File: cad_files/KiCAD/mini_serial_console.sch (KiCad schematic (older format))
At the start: 45 parts, among them J1 Screw_Terminal_1x02, J2 Screw_Terminal_1x03, J3 Screw_Terminal_1x03, J4 Screw_Terminal_1x07, Q1 BC559, Q2 BC548, Q3 BC109, U1 HD44780 compatible LCD, U2 Raspberry Pi Pico

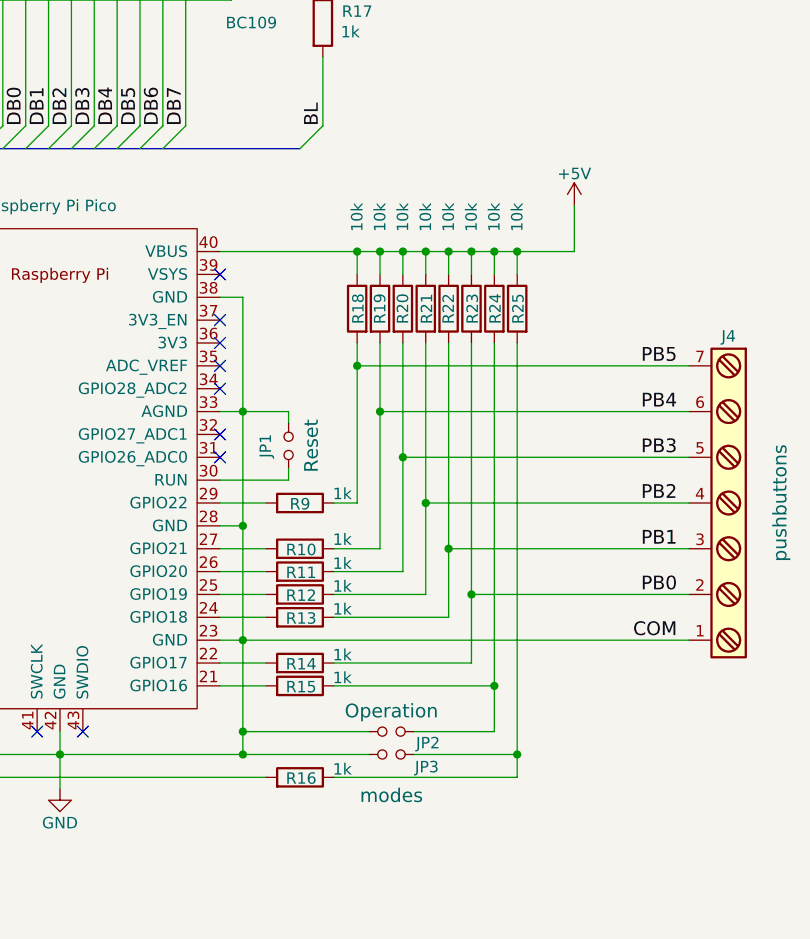
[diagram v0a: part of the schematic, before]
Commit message: 221115
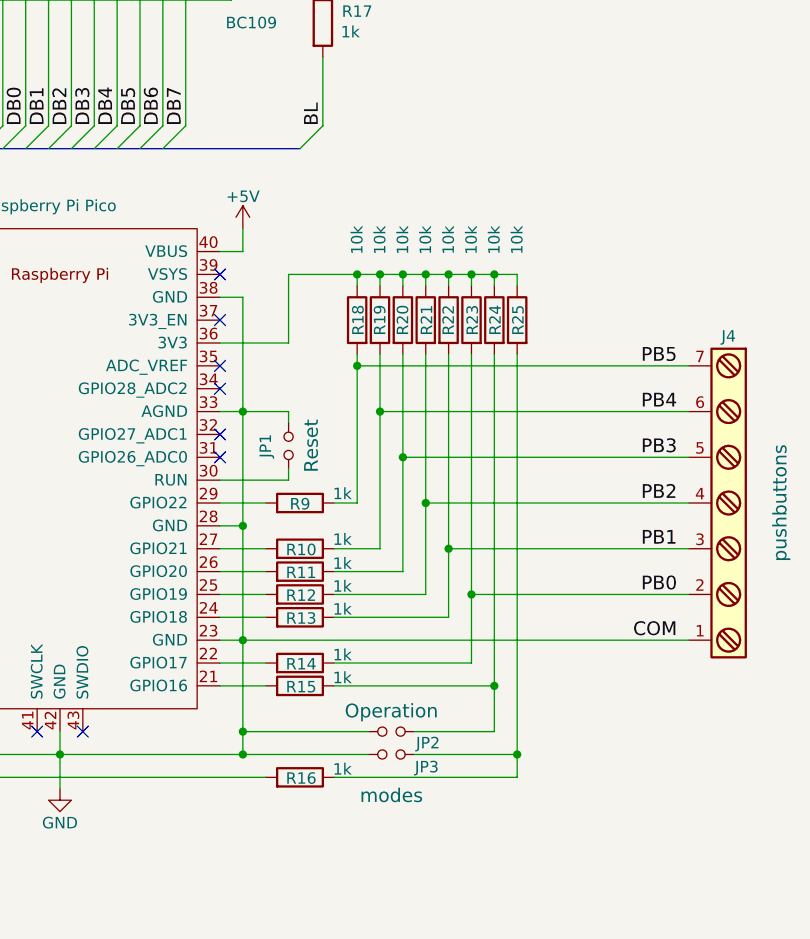
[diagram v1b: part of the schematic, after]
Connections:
- net +5V: no longer R18.1, R19.1, R20.1, R21.1, R22.1, R23.1, R24.1, R25.1
- net at U2.36 (3V3): now also R18.1, R19.1, R20.1, R21.1, R22.1, R23.1, R24.1, R25.1
- no-connect marks 9 -> 8
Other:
- moved on the sheet: R18, R19, R20, R21, R22, R23, R24, R25
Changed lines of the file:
@@
 Entry Wire Line
 	6300 3300 6400 3200
-NoConn ~ 7550 4150
 NoConn ~ 7550 4050
 NoConn ~ 7550 3850
@@
 Connection ~ 4650 4150
 Wire Wire Line
-	7650 3950 7650 5950
+	7650 5950 7650 3950
 Wire Wire Line
 	7650 4950 7550 4950
@@
 $EndComp
 Wire Wire Line
-	8150 3850 8150 3750
-Wire Wire Line
-	8350 4150 8350 5150
-Wire Wire Line
-	8250 4150 8250 5050
-Wire Wire Line
-	8150 4150 8150 4850
-Connection ~ 8150 3750
-Connection ~ 8350 3750
-Wire Wire Line
-	8350 3850 8350 3750
-Connection ~ 8250 3750
-Wire Wire Line
-	8250 3850 8250 3750
+	8150 3900 8150 3850
+Wire Wire Line
+	8350 4200 8350 5150
+Wire Wire Line
+	8250 4200 8250 5050
+Wire Wire Line
+	8150 4200 8150 4850
+Connection ~ 8150 3850
+Connection ~ 8350 3850
+Wire Wire Line
+	8350 3900 8350 3850
+Connection ~ 8250 3850
+Wire Wire Line
+	8250 3900 8250 3850
 $Comp
 L R R20
 U 1 1 63354AD8
-P 8350 4000
-F 0 "R20" V 8350 4000 50  0000 C CNN
+P 8350 4050
+F 0 "R20" V 8350 4050 50  0000 C CNN
 F 1 "10k" V 8350 4400 50  0000 C CNN
-F 2 "Resistors_THT:R_Axial_DIN0309_L9.0mm_D3.2mm_P5.08mm_Vertical" V 8280 4000 50  0001 C CNN
-F 3 "" H 8350 4000 50  0000 C CNN
-	1    8350 4000
+F 2 "Resistors_THT:R_Axial_DIN0309_L9.0mm_D3.2mm_P5.08mm_Vertical" V 8280 4050 50  0001 C CNN
+F 3 "" H 8350 4050 50  0000 C CNN
+	1    8350 4050
 	1    0    0    -1
 $EndComp
@@
 L R R18
 U 1 1 63356FF1
-P 8150 4000
-F 0 "R18" V 8145 4000 50  0000 C CNN
+P 8150 4050
+F 0 "R18" V 8145 4050 50  0000 C CNN
 F 1 "10k" V 8150 4400 50  0000 C CNN
-F 2 "Resistors_THT:R_Axial_DIN0309_L9.0mm_D3.2mm_P5.08mm_Vertical" V 8080 4000 50  0001 C CNN
-F 3 "" H 8150 4000 50  0000 C CNN
-	1    8150 4000
+F 2 "Resistors_THT:R_Axial_DIN0309_L9.0mm_D3.2mm_P5.08mm_Vertical" V 8080 4050 50  0001 C CNN
+F 3 "" H 8150 4050 50  0000 C CNN
+	1    8150 4050
 	-1   0    0    -1
 $EndComp
@@
 L R R19
 U 1 1 63356FDE
-P 8250 4000
-F 0 "R19" V 8250 4000 50  0000 C CNN
+P 8250 4050
+F 0 "R19" V 8250 4050 50  0000 C CNN
 F 1 "10k" V 8250 4400 50  0000 C CNN
-F 2 "Resistors_THT:R_Axial_DIN0309_L9.0mm_D3.2mm_P5.08mm_Vertical" V 8180 4000 50  0001 C CNN
-F 3 "" H 8250 4000 50  0000 C CNN
-	1    8250 4000
-	1    0    0    -1
-$EndComp
-Wire Wire Line
-	9100 3750 9100 3550
+F 2 "Resistors_THT:R_Axial_DIN0309_L9.0mm_D3.2mm_P5.08mm_Vertical" V 8180 4050 50  0001 C CNN
+F 3 "" H 8250 4050 50  0000 C CNN
+	1    8250 4050
+	1    0    0    -1
+$EndComp
+Wire Wire Line
+	7650 3750 7650 3650
 $Comp
 L +5V #PWR010
 U 1 1 6334DE99
-P 9100 3550
-F 0 "#PWR010" H 9100 3400 50  0001 C CNN
-F 1 "+5V" H 9100 3690 50  0000 C CNN
-F 2 "" H 9100 3550 50  0000 C CNN
-F 3 "" H 9100 3550 50  0000 C CNN
-	1    9100 3550
+P 7650 3650
+F 0 "#PWR010" H 7650 3500 50  0001 C CNN
+F 1 "+5V" H 7650 3790 50  0000 C CNN
+F 2 "" H 7650 3650 50  0000 C CNN
+F 3 "" H 7650 3650 50  0000 C CNN
+	1    7650 3650
 	1    0    0    -1
 $EndComp
@@
 L R R21
 U 1 1 63354AD2
-P 8450 4000
-F 0 "R21" V 8445 4000 50  0000 C CNN
+P 8450 4050
+F 0 "R21" V 8445 4050 50  0000 C CNN
 F 1 "10k" V 8350 4400 50  0000 C CNN
-F 2 "Resistors_THT:R_Axial_DIN0309_L9.0mm_D3.2mm_P5.08mm_Vertical" V 8380 4000 50  0001 C CNN
-F 3 "" H 8450 4000 50  0000 C CNN
-	1    8450 4000
+F 2 "Resistors_THT:R_Axial_DIN0309_L9.0mm_D3.2mm_P5.08mm_Vertical" V 8380 4050 50  0001 C CNN
+F 3 "" H 8450 4050 50  0000 C CNN
+	1    8450 4050
 	-1   0    0    -1
 $EndComp
@@
 L R R22
 U 1 1 633680FD
-P 8550 4000
-F 0 "R22" V 8550 4000 50  0000 C CNN
+P 8550 4050
+F 0 "R22" V 8550 4050 50  0000 C CNN
 F 1 "10k" V 8450 4400 50  0000 C CNN
-F 2 "Resistors_THT:R_Axial_DIN0309_L9.0mm_D3.2mm_P5.08mm_Vertical" V 8480 4000 50  0001 C CNN
-F 3 "" H 8550 4000 50  0000 C CNN
-	1    8550 4000
+F 2 "Resistors_THT:R_Axial_DIN0309_L9.0mm_D3.2mm_P5.08mm_Vertical" V 8480 4050 50  0001 C CNN
+F 3 "" H 8550 4050 50  0000 C CNN
+	1    8550 4050
 	1    0    0    -1
 $EndComp
@@
 L R R23
 U 1 1 63366A0E
-P 8650 4000
-F 0 "R23" V 8645 4000 50  0000 C CNN
+P 8650 4050
+F 0 "R23" V 8645 4050 50  0000 C CNN
 F 1 "10k" V 8650 4400 50  0000 C CNN
-F 2 "Resistors_THT:R_Axial_DIN0309_L9.0mm_D3.2mm_P5.08mm_Vertical" V 8580 4000 50  0001 C CNN
-F 3 "" H 8650 4000 50  0000 C CNN
-	1    8650 4000
+F 2 "Resistors_THT:R_Axial_DIN0309_L9.0mm_D3.2mm_P5.08mm_Vertical" V 8580 4050 50  0001 C CNN
+F 3 "" H 8650 4050 50  0000 C CNN
+	1    8650 4050
 	-1   0    0    -1
 $EndComp
@@
 L R R24
 U 1 1 633736D1
-P 8750 4000
-F 0 "R24" V 8745 4000 50  0000 C CNN
+P 8750 4050
+F 0 "R24" V 8745 4050 50  0000 C CNN
 F 1 "10k" V 8750 4400 50  0000 C CNN
-F 2 "Resistors_THT:R_Axial_DIN0309_L9.0mm_D3.2mm_P5.08mm_Vertical" V 8680 4000 50  0001 C CNN
-F 3 "" H 8750 4000 50  0000 C CNN
-	1    8750 4000
+F 2 "Resistors_THT:R_Axial_DIN0309_L9.0mm_D3.2mm_P5.08mm_Vertical" V 8680 4050 50  0001 C CNN
+F 3 "" H 8750 4050 50  0000 C CNN
+	1    8750 4050
 	-1   0    0    -1
 $EndComp
@@
 L R R25
 U 1 1 63373754
-P 8850 4000
-F 0 "R25" V 8845 4000 50  0000 C CNN
+P 8850 4050
+F 0 "R25" V 8845 4050 50  0000 C CNN
 F 1 "10k" V 8850 4400 50  0000 C CNN
-F 2 "Resistors_THT:R_Axial_DIN0309_L9.0mm_D3.2mm_P5.08mm_Vertical" V 8780 4000 50  0001 C CNN
-F 3 "" H 8850 4000 50  0000 C CNN
-	1    8850 4000
+F 2 "Resistors_THT:R_Axial_DIN0309_L9.0mm_D3.2mm_P5.08mm_Vertical" V 8780 4050 50  0001 C CNN
+F 3 "" H 8850 4050 50  0000 C CNN
+	1    8850 4050
 	-1   0    0    -1
 $EndComp
 Wire Wire Line
-	7550 3750 9100 3750
-Wire Wire Line
-	8650 3750 8650 3850
-Wire Wire Line
-	8450 3750 8450 3850
-Connection ~ 8450 3750
-Wire Wire Line
-	8550 3750 8550 3850
-Connection ~ 8550 3750
-Wire Wire Line
-	8450 4150 8450 5250
-Wire Wire Line
-	8550 4150 8550 5350
-Wire Wire Line
-	8650 4150 8650 5550
-Wire Wire Line
-	8750 4150 8750 5850
-Wire Wire Line
-	8850 4150 8850 6050
-Wire Wire Line
-	8750 3750 8750 3850
-Connection ~ 8650 3750
-Wire Wire Line
-	8850 3750 8850 3850
-Connection ~ 8750 3750
-Connection ~ 8850 3750
+	8650 3850 8650 3900
+Wire Wire Line
+	8450 3850 8450 3900
+Connection ~ 8450 3850
+Wire Wire Line
+	8550 3850 8550 3900
+Connection ~ 8550 3850
+Wire Wire Line
+	8450 4200 8450 5250
+Wire Wire Line
+	8550 4200 8550 5350
+Wire Wire Line
+	8650 4200 8650 5550
+Wire Wire Line
+	8750 4200 8750 5850
+Wire Wire Line
+	8850 4200 8850 6050
+Wire Wire Line
+	8750 3850 8750 3900
+Connection ~ 8650 3850
+Wire Wire Line
+	8850 3850 8850 3900
+Connection ~ 8750 3850
 Wire Wire Line
 	6200 1800 6200 1900
@@
 Wire Notes Line
 	6200 7500 6200 6950
+Wire Wire Line
+	7850 3850 8850 3850
+Wire Wire Line
+	7850 3850 7850 4150
+Wire Wire Line
+	7850 4150 7550 4150
+Wire Wire Line
+	7550 3750 7650 3750
 $EndSCHEMATC
